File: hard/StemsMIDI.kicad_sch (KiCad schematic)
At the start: 190 parts, among them SW1 SW_SPST, SW10 SW_SPST, SW11 SW_SPST, SW12 SW_SPST, SW13 SW_SPST, SW14 SW_SPST, SW15 SW_SPST, SW16 SW_SPST, SW17 SW_SPST, SW18 SW_SPST, SW19 SW_SPST, SW2 SW_SPST, SW20 SW_SPST, SW21 SW_SPST, SW22 SW_SPST, SW23 SW_SPST, SW24 SW_SPST, SW3 SW_SPST, SW4 SW_SPST, SW5 SW_SPST, SW6 SW_SPST, SW7 SW_SPST, SW8 SW_SPST, SW9 SW_SPST, U1 74HC4051, U2 74HC4051, U3 74HC4051, U4 74HC165, U5 74HC165, U6 74HC165, U7 MOUDLE-SEEEDUINO-XIAO

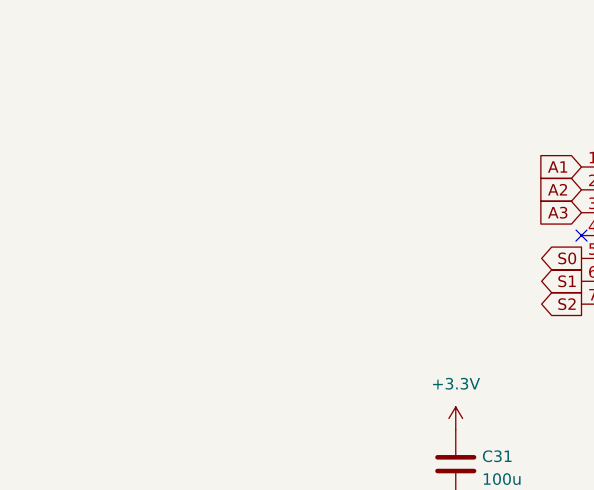
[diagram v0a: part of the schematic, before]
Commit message: modify for rev 1.1
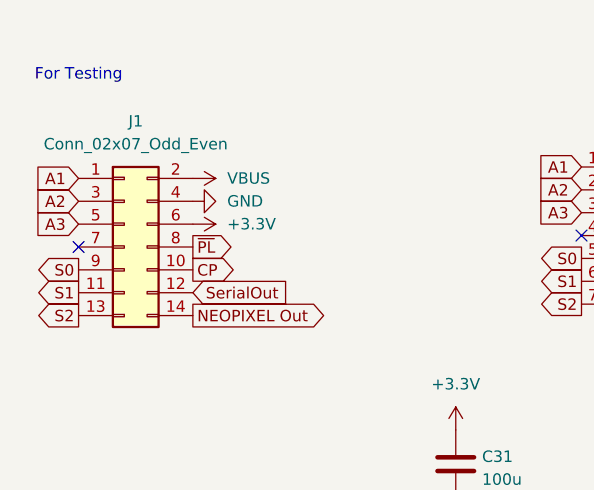
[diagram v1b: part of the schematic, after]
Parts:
- added J1: Conn_02x07_Odd_Even, my_footprint:PinSocket_2x07_P2.54mm_Vertical_Flipped, symbol Connector_Generic:Conn_02x07_Odd_Even
- RV11, RV14, RV17, RV2, RV20, RV23, RV5, RV8: LCSC C470315 -> C470304
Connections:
- net +3.3V: now also J1.6 (Pin_6)
- net A1: now also J1.1 (Pin_1)
- net A2: now also J1.3 (Pin_3)
- net A3: now also J1.5 (Pin_5)
- net CP: now also J1.10 (Pin_10)
- net GND: now also J1.4 (Pin_4)
- net NEOPIXEL Out: now also J1.14 (Pin_14)
- net S0: now also J1.9 (Pin_9)
- net S1: now also J1.11 (Pin_11)
- net S2: now also J1.13 (Pin_13)
- net SerialOut: now also J1.12 (Pin_12)
- net VBUS: now also J1.2 (Pin_2)
- net ~{PL}: now also J1.8 (Pin_8)
- no-connect marks 5 -> 6
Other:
- note added: "For Testing"

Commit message: [hard] Correct LCSC #
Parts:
- RV1, RV10, RV12, RV13, RV15, RV16, RV18, RV19, RV21, RV22, RV24, RV3, RV4, RV6, RV7, RV9: LCSC C470315 -> C470304
- RV11, RV14, RV17, RV2, RV20, RV23, RV5, RV8: LCSC C470304 -> C470315
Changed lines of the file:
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@@
 			)
 		)
-		(property "LCSC" "C470315"
+		(property "LCSC" "C470304"
 			(at 92.71 304.8 0)
 			(effects
@@
 			)
 		)
-		(property "LCSC" "C470304"
+		(property "LCSC" "C470315"
 			(at 455.93 330.2 0)
 			(effects
@@
 			)
 		)
-		(property "LCSC" "C470315"
+		(property "LCSC" "C470304"
 			(at 386.08 354.33 0)
 			(effects
@@
 			)
 		)
-		(property "LCSC" "C470304"
+		(property "LCSC" "C470315"
 			(at 162.56 304.8 0)
 			(effects
@@
 			)
 		)
-		(property "LCSC" "C470304"
+		(property "LCSC" "C470315"
 			(at 162.56 379.73 0)
 			(effects
@@
 			)
 		)
-		(property "LCSC" "C470315"
+		(property "LCSC" "C470304"
 			(at 386.08 379.73 0)
 			(effects
@@
 			)
 		)
-		(property "LCSC" "C470315"
+		(property "LCSC" "C470304"
 			(at 231.14 304.8 0)
 			(effects
@@
 			)
 		)
-		(property "LCSC" "C470304"
+		(property "LCSC" "C470315"
 			(at 162.56 354.33 0)
 			(effects
@@
 			)
 		)
-		(property "LCSC" "C470304"
+		(property "LCSC" "C470315"
 			(at 162.56 330.2 0)
 			(effects
@@
 			)
 		)
-		(property "LCSC" "C470315"
+		(property "LCSC" "C470304"
 			(at 92.71 354.33 0)
 			(effects
@@
 			)
 		)
-		(property "LCSC" "C470304"
+		(property "LCSC" "C470315"
 			(at 455.93 304.8 0)
 			(effects
@@
 			)
 		)
-		(property "LCSC" "C470304"
+		(property "LCSC" "C470315"
 			(at 455.93 354.33 0)
 			(effects
@@
 			)
 		)
-		(property "LCSC" "C470315"
+		(property "LCSC" "C470304"
 			(at 524.51 379.73 0)
 			(effects
@@
 			)
 		)
-		(property "LCSC" "C470315"
+		(property "LCSC" "C470304"
 			(at 231.14 354.33 0)
 			(effects
@@
 			)
 		)
-		(property "LCSC" "C470304"
+		(property "LCSC" "C470315"
 			(at 455.93 379.73 0)
 			(effects
@@
 			)
 		)
-		(property "LCSC" "C470315"
+		(property "LCSC" "C470304"
 			(at 524.51 304.8 0)
 			(effects
@@
 			)
 		)
-		(property "LCSC" "C470315"
+		(property "LCSC" "C470304"
 			(at 92.71 379.73 0)
 			(effects
@@
 			)
 		)
-		(property "LCSC" "C470315"
+		(property "LCSC" "C470304"
 			(at 524.51 354.33 0)
 			(effects
@@
 			)
 		)
-		(property "LCSC" "C470315"
+		(property "LCSC" "C470304"
 			(at 386.08 330.2 0)
 			(effects
@@
 			)
 		)
-		(property "LCSC" "C470315"
+		(property "LCSC" "C470304"
 			(at 524.51 330.2 0)
 			(effects
@@
 			)
 		)
-		(property "LCSC" "C470315"
+		(property "LCSC" "C470304"
 			(at 386.08 304.8 0)
 			(effects
@@
 			)
 		)
-		(property "LCSC" "C470315"
+		(property "LCSC" "C470304"
 			(at 92.71 330.2 0)
 			(effects
@@
 			)
 		)
-		(property "LCSC" "C470315"
+		(property "LCSC" "C470304"
 			(at 231.14 379.73 0)
 			(effects
@@
 			)
 		)
-		(property "LCSC" "C470315"
+		(property "LCSC" "C470304"
 			(at 231.14 330.2 0)
 			(effects

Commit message: [case] reorganize, rename case and pcb files
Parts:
- C31: LCSC C312983 -> C15008
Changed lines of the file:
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@@
 (kicad_sch
-	(version 20231120)
+	(version 20250114)
 	(generator "eeschema")
-	(generator_version "8.0")
+	(generator_version "9.0")
 	(paper "A1")
+	(text "For Testing"
+		(exclude_from_sim no)
+		(at 69.85 82.55 0)
+		(effects
+			(font
+				(size 1.27 1.27)
+			)
+		)
+	)
 	(junction
 		(at 92.71 417.83)
@@
 		)
 	)
-	(text "For Testing"
-		(exclude_from_sim no)
-		(at 69.85 82.55 0)
-		(effects
-			(font
-				(size 1.27 1.27)
-			)
-		)
-	)
 	(global_label "SerialOut"
 		(shape output)
@@
 			)
 		)
-		(property "LCSC" "C312983"
+		(property "LCSC" "C15008"
 			(at 111.76 125.73 0)
 			(effects
@@
 		)
 	)
+	(embedded_fonts no)
 )
